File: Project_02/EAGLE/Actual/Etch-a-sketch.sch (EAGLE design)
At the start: 24 parts, among them J1 292303-1, J2 SPI_LCD, SW1 PUSH_BUTTON, SW2 PUSH_BUTTON, U1 POCKETBEAGLE

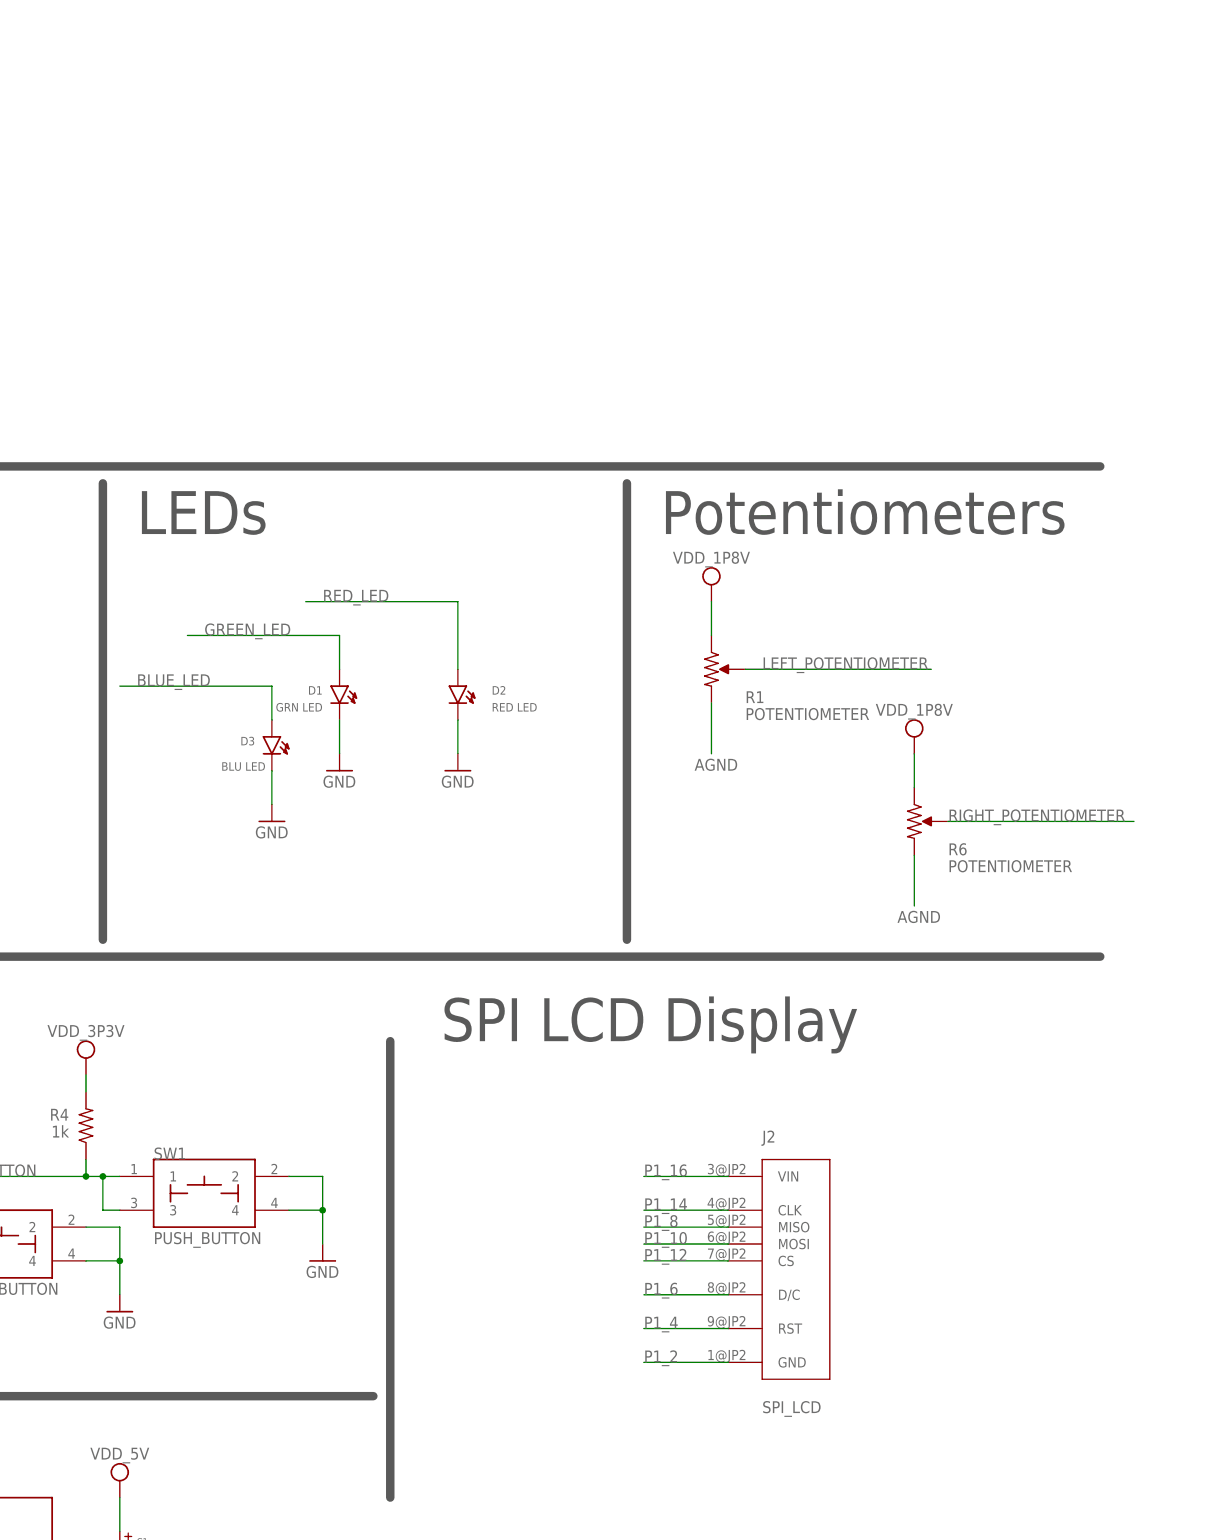
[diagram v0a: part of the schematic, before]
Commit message: etch the sketch
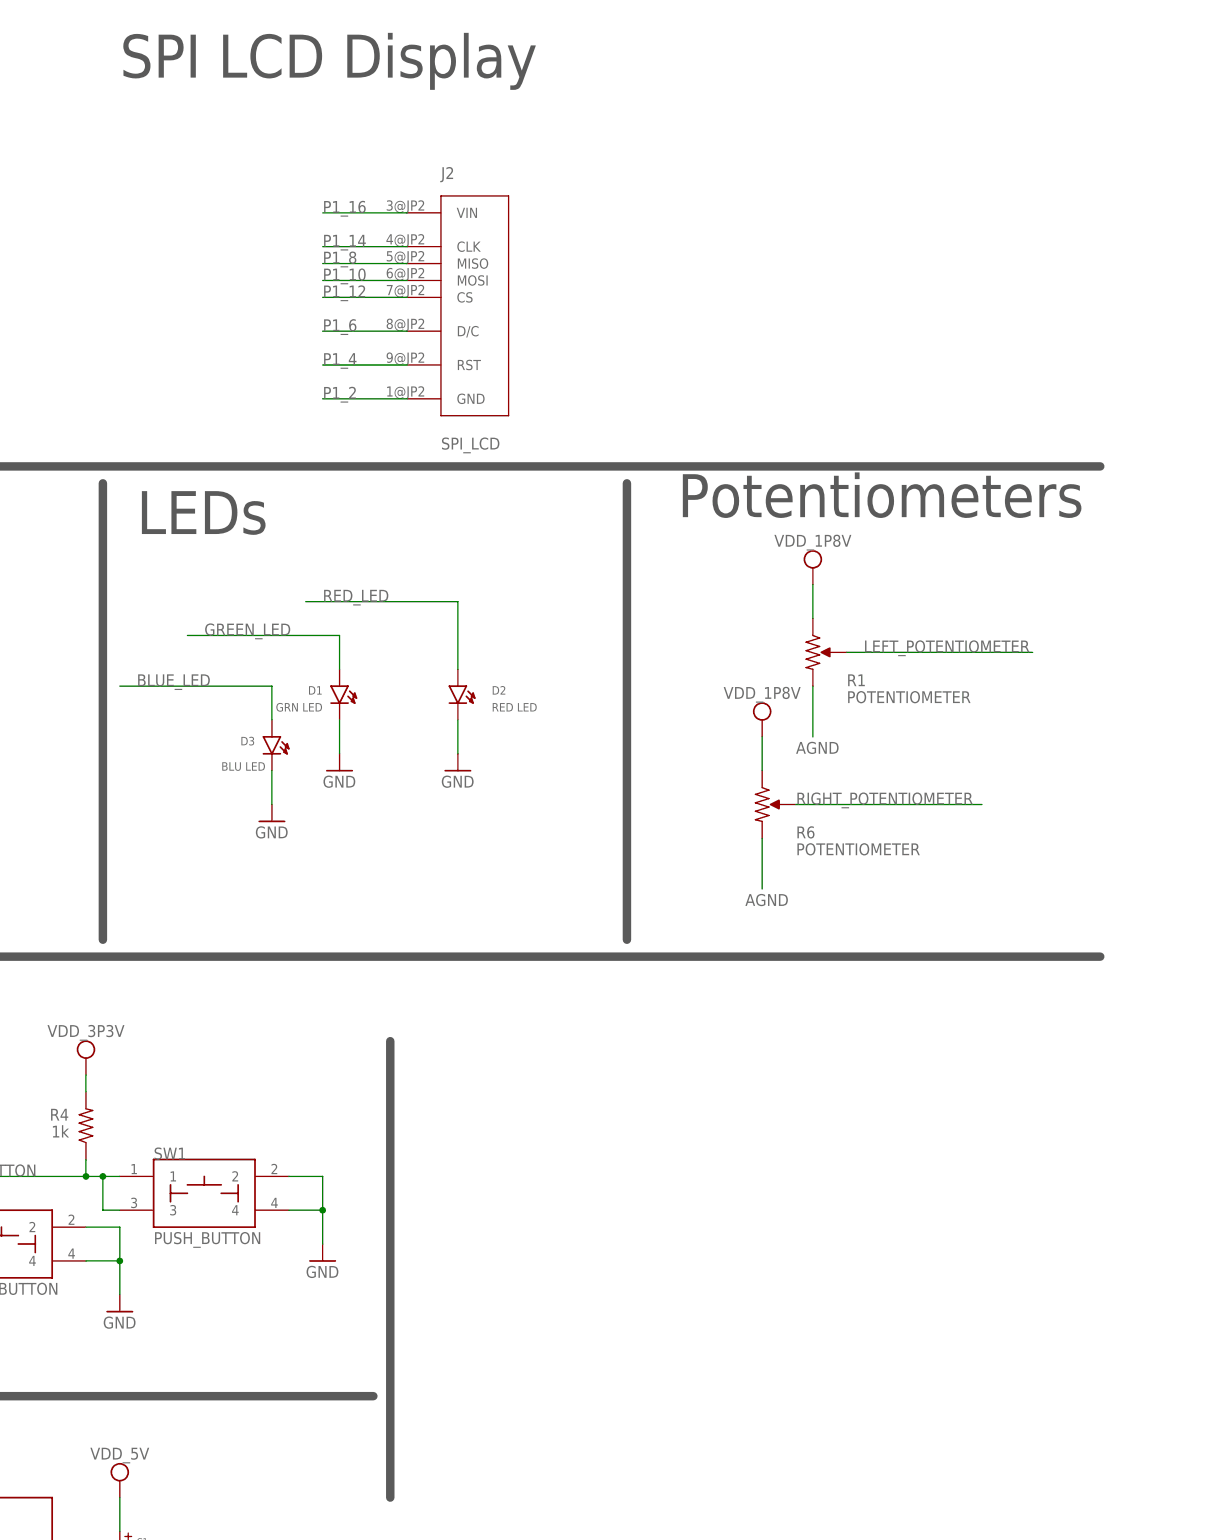
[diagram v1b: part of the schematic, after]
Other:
- moved on the sheet: J2, R1, R6
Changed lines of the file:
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@@
 <wire x1="304.8" y1="114.3" x2="304.8" y2="182.88" width="1.27" layer="97"/>
 <text x="231.14" y="175.26" size="6.4516" layer="97">LEDs</text>
-<text x="309.88" y="175.26" size="6.4516" layer="97">Potentiometers</text>
-<text x="276.86" y="99.06" size="6.4516" layer="97">SPI LCD Display</text>
+<text x="312.42" y="177.8" size="6.4516" layer="97">Potentiometers</text>
+<text x="228.6" y="243.84" size="6.4516" layer="97">SPI LCD Display</text>
 <text x="177.8" y="99.06" size="6.4516" layer="97">Button</text>
 <text x="12.7" y="241.3" size="6.4516" layer="97">PocketBeagle</text>
@@
 <text x="243.84" y="139.7" size="1.27" layer="95">BLU LED</text>
 <text x="-309.88" y="15.24" size="1.778" layer="95">RIGHT_POTENTIOMETER</text>
-<text x="353.06" y="132.08" size="1.778" layer="95">RIGHT_POTENTIOMETER</text>
+<text x="330.2" y="134.62" size="1.778" layer="95">RIGHT_POTENTIOMETER</text>
 <text x="170.18" y="71.12" size="1.778" layer="95">RIGHT_BUTTON</text>
-<text x="307.34" y="78.74" size="1.778" layer="95">P1_16</text>
-<text x="307.34" y="73.66" size="1.778" layer="95">P1_14</text>
-<text x="307.34" y="71.12" size="1.778" layer="95">P1_8</text>
-<text x="307.34" y="68.58" size="1.778" layer="95">P1_10</text>
-<text x="307.34" y="66.04" size="1.778" layer="95">P1_12</text>
-<text x="307.34" y="60.96" size="1.778" layer="95">P1_6</text>
-<text x="307.34" y="55.88" size="1.778" layer="95">P1_4</text>
-<text x="307.34" y="50.8" size="1.778" layer="95">P1_2</text>
+<text x="259.08" y="223.52" size="1.778" layer="95">P1_16</text>
+<text x="259.08" y="218.44" size="1.778" layer="95">P1_14</text>
+<text x="259.08" y="215.9" size="1.778" layer="95">P1_8</text>
+<text x="259.08" y="213.36" size="1.778" layer="95">P1_10</text>
+<text x="259.08" y="210.82" size="1.778" layer="95">P1_12</text>
+<text x="259.08" y="205.74" size="1.778" layer="95">P1_6</text>
+<text x="259.08" y="200.66" size="1.778" layer="95">P1_4</text>
+<text x="259.08" y="195.58" size="1.778" layer="95">P1_2</text>
 </plain>
 <instances>
@@
 <attribute name="VALUE" x="259.08" y="149.86" size="1.27" layer="96" rot="R180"/>
 </instance>
-<instance part="R1" gate="G$1" x="317.5" y="154.94" smashed="yes">
-<attribute name="NAME" x="322.58" y="149.86" size="1.778" layer="95"/>
-<attribute name="VALUE" x="322.58" y="147.32" size="1.778" layer="96"/>
+<instance part="R1" gate="G$1" x="332.74" y="157.48" smashed="yes">
+<attribute name="NAME" x="337.82" y="152.4" size="1.778" layer="95"/>
+<attribute name="VALUE" x="337.82" y="149.86" size="1.778" layer="96"/>
 </instance>
 <instance part="SW1" gate="G$1" x="241.3" y="76.2" smashed="yes">
@@
 <attribute name="VALUE" x="276.86" y="137.16" size="1.778" layer="96"/>
 </instance>
-<instance part="SUPPLY5" gate="G$1" x="317.5" y="167.64" smashed="yes">
-<attribute name="VALUE" x="317.5" y="171.704" size="1.778" layer="96" align="center"/>
+<instance part="SUPPLY5" gate="G$1" x="332.74" y="170.18" smashed="yes">
+<attribute name="VALUE" x="332.74" y="174.244" size="1.778" layer="96" align="center"/>
 </instance>
 <instance part="GND7" gate="1" x="259.08" y="66.04" smashed="yes">
@@
 <attribute name="VALUE" x="226.06" y="7.62" size="1.778" layer="96"/>
 </instance>
-<instance part="J2" gate="G$1" x="320.04" y="58.42" smashed="yes">
-<attribute name="NAME" x="325.12" y="83.82" size="1.778" layer="95"/>
-<attribute name="VALUE" x="325.12" y="43.18" size="1.778" layer="95"/>
+<instance part="J2" gate="G$1" x="271.78" y="203.2" smashed="yes">
+<attribute name="NAME" x="276.86" y="228.6" size="1.778" layer="95"/>
+<attribute name="VALUE" x="276.86" y="187.96" size="1.778" layer="95"/>
 </instance>
 <instance part="D3" gate="G$1" x="251.46" y="144.78" smashed="yes" rot="R270">
@@
 <attribute name="VALUE" x="248.92" y="129.54" size="1.778" layer="96"/>
 </instance>
-<instance part="R6" gate="G$1" x="347.98" y="132.08" smashed="yes">
-<attribute name="NAME" x="353.06" y="127" size="1.778" layer="95"/>
-<attribute name="VALUE" x="353.06" y="124.46" size="1.778" layer="96"/>
-</instance>
-<instance part="SUPPLY6" gate="G$1" x="347.98" y="144.78" smashed="yes">
-<attribute name="VALUE" x="347.98" y="148.844" size="1.778" layer="96" align="center"/>
+<instance part="R6" gate="G$1" x="325.12" y="134.62" smashed="yes">
+<attribute name="NAME" x="330.2" y="129.54" size="1.778" layer="95"/>
+<attribute name="VALUE" x="330.2" y="127" size="1.778" layer="96"/>
+</instance>
+<instance part="SUPPLY6" gate="G$1" x="325.12" y="147.32" smashed="yes">
+<attribute name="VALUE" x="325.12" y="151.384" size="1.778" layer="96" align="center"/>
 </instance>
 <instance part="SW2" gate="G$1" x="210.82" y="68.58" smashed="yes">
@@
 <pinref part="R1" gate="G$1" pin="CCW"/>
 <pinref part="SUPPLY5" gate="G$1" pin="VDD_1P8V"/>
-<wire x1="317.5" y1="160.02" x2="317.5" y2="165.1" width="0.1524" layer="91"/>
+<wire x1="332.74" y1="162.56" x2="332.74" y2="167.64" width="0.1524" layer="91"/>
 </segment>
 <segment>
@@
 <pinref part="R6" gate="G$1" pin="CCW"/>
 <pinref part="SUPPLY6" gate="G$1" pin="VDD_1P8V"/>
-<wire x1="347.98" y1="137.16" x2="347.98" y2="142.24" width="0.1524" layer="91"/>
+<wire x1="325.12" y1="139.7" x2="325.12" y2="144.78" width="0.1524" layer="91"/>
 </segment>
 </net>
@@
 <segment>
 <pinref part="R1" gate="G$1" pin="CW"/>
-<wire x1="317.5" y1="149.86" x2="317.5" y2="142.24" width="0.1524" layer="91"/>
-<label x="314.96" y="139.7" size="1.778" layer="95"/>
+<wire x1="332.74" y1="152.4" x2="332.74" y2="144.78" width="0.1524" layer="91"/>
+<label x="330.2" y="142.24" size="1.778" layer="95"/>
 </segment>
 <segment>
@@
 <segment>
 <pinref part="R6" gate="G$1" pin="CW"/>
-<wire x1="347.98" y1="127" x2="347.98" y2="119.38" width="0.1524" layer="91"/>
-<label x="345.44" y="116.84" size="1.778" layer="95"/>
+<wire x1="325.12" y1="129.54" x2="325.12" y2="121.92" width="0.1524" layer="91"/>
+<label x="322.58" y="119.38" size="1.778" layer="95"/>
 </segment>
 </net>
@@
 <segment>
 <pinref part="R1" gate="G$1" pin="S"/>
-<wire x1="322.58" y1="154.94" x2="350.52" y2="154.94" width="0.1524" layer="91"/>
-<label x="325.12" y="154.94" size="1.778" layer="95"/>
+<wire x1="337.82" y1="157.48" x2="365.76" y2="157.48" width="0.1524" layer="91"/>
+<label x="340.36" y="157.48" size="1.778" layer="95"/>
 </segment>
 <segment>
 <pinref part="R6" gate="G$1" pin="S"/>
-<wire x1="353.06" y1="132.08" x2="381" y2="132.08" width="0.1524" layer="91"/>
+<wire x1="330.2" y1="134.62" x2="358.14" y2="134.62" width="0.1524" layer="91"/>
 </segment>
 </net>
@@
 <segment>
 <pinref part="J2" gate="G$1" pin="VIN"/>
-<wire x1="320.04" y1="78.74" x2="307.34" y2="78.74" width="0.1524" layer="91"/>
+<wire x1="271.78" y1="223.52" x2="259.08" y2="223.52" width="0.1524" layer="91"/>
 </segment>
 </net>
 <net name="N$2" class="0">
 <segment>
-<wire x1="320.04" y1="73.66" x2="307.34" y2="73.66" width="0.1524" layer="91"/>
+<wire x1="271.78" y1="218.44" x2="259.08" y2="218.44" width="0.1524" layer="91"/>
 <pinref part="J2" gate="G$1" pin="CLK"/>
 </segment>
@@
 <net name="N$3" class="0">
 <segment>
-<wire x1="320.04" y1="71.12" x2="307.34" y2="71.12" width="0.1524" layer="91"/>
+<wire x1="271.78" y1="215.9" x2="259.08" y2="215.9" width="0.1524" layer="91"/>
 <pinref part="J2" gate="G$1" pin="MISO"/>
 </segment>
@@
 <net name="N$4" class="0">
 <segment>
-<wire x1="320.04" y1="68.58" x2="307.34" y2="68.58" width="0.1524" layer="91"/>
+<wire x1="271.78" y1="213.36" x2="259.08" y2="213.36" width="0.1524" layer="91"/>
 <pinref part="J2" gate="G$1" pin="MOSI"/>
 </segment>
@@
 <net name="N$5" class="0">
 <segment>
-<wire x1="320.04" y1="66.04" x2="307.34" y2="66.04" width="0.1524" layer="91"/>
+<wire x1="271.78" y1="210.82" x2="259.08" y2="210.82" width="0.1524" layer="91"/>
 <pinref part="J2" gate="G$1" pin="CS"/>
 </segment>
@@
 <net name="N$6" class="0">
 <segment>
-<wire x1="320.04" y1="60.96" x2="307.34" y2="60.96" width="0.1524" layer="91"/>
+<wire x1="271.78" y1="205.74" x2="259.08" y2="205.74" width="0.1524" layer="91"/>
 <pinref part="J2" gate="G$1" pin="D/C"/>
 </segment>
@@
 <net name="N$7" class="0">
 <segment>
-<wire x1="320.04" y1="55.88" x2="307.34" y2="55.88" width="0.1524" layer="91"/>
+<wire x1="271.78" y1="200.66" x2="259.08" y2="200.66" width="0.1524" layer="91"/>
 <pinref part="J2" gate="G$1" pin="RST"/>
 </segment>
@@
 <net name="N$8" class="0">
 <segment>
-<wire x1="320.04" y1="50.8" x2="307.34" y2="50.8" width="0.1524" layer="91"/>
+<wire x1="271.78" y1="195.58" x2="259.08" y2="195.58" width="0.1524" layer="91"/>
 <pinref part="J2" gate="G$1" pin="GND"/>
 </segment>
